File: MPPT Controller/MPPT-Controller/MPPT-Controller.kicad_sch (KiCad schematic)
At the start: 48 parts, among them J1 Conn_01x02_Pin, J2 Conn_01x02_Pin, J3 Conn_01x02_Pin, J4 USB_C_Receptacle_PowerOnly_6P, K1 JQC-3FF-005-1Z, Q1 BC817, U1 ADS1115IDGS, U2 ESP32-WROOM-32D

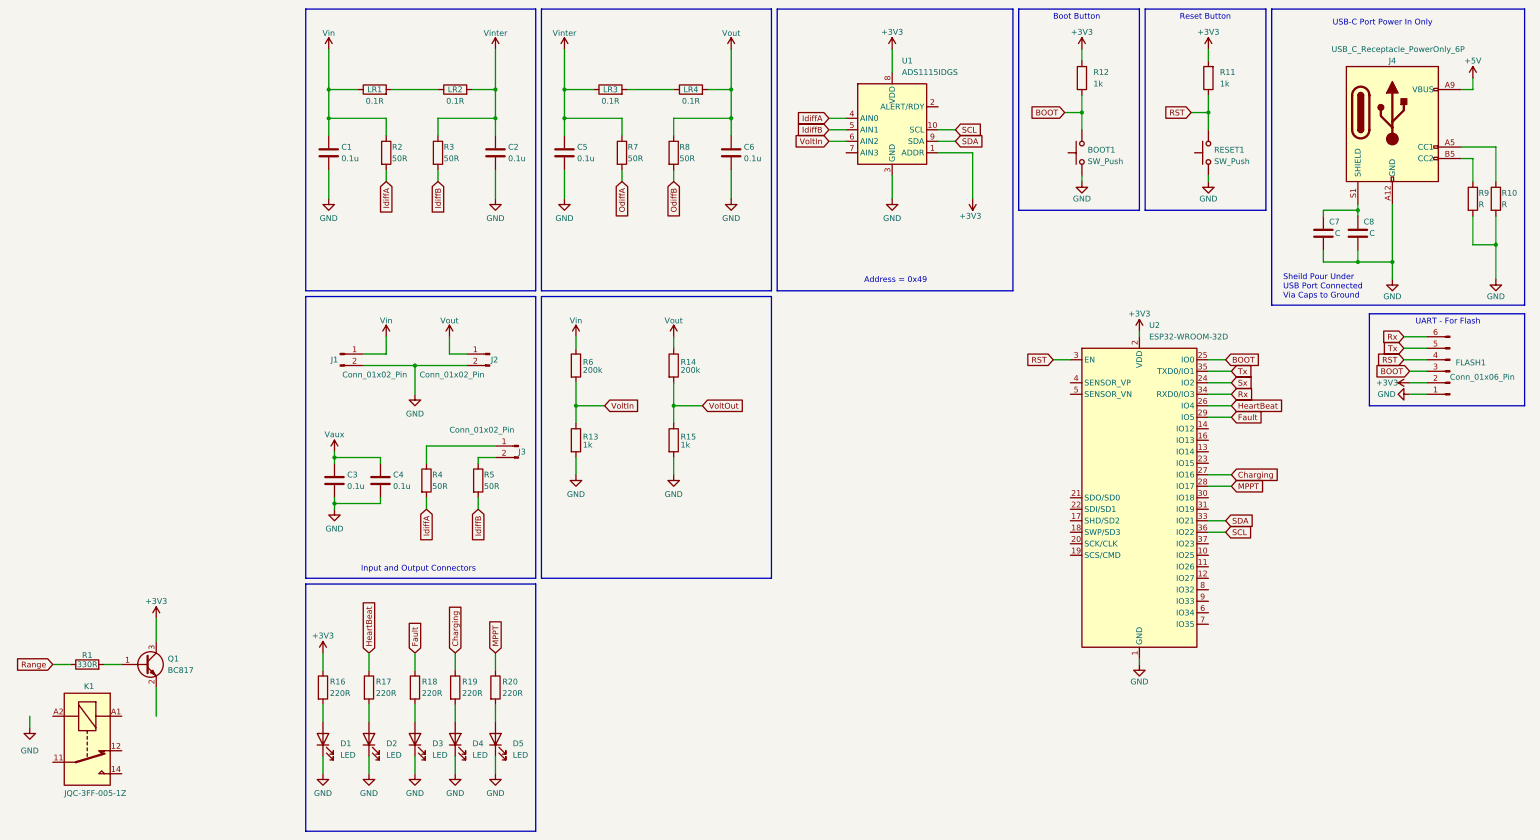
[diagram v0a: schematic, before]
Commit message: add
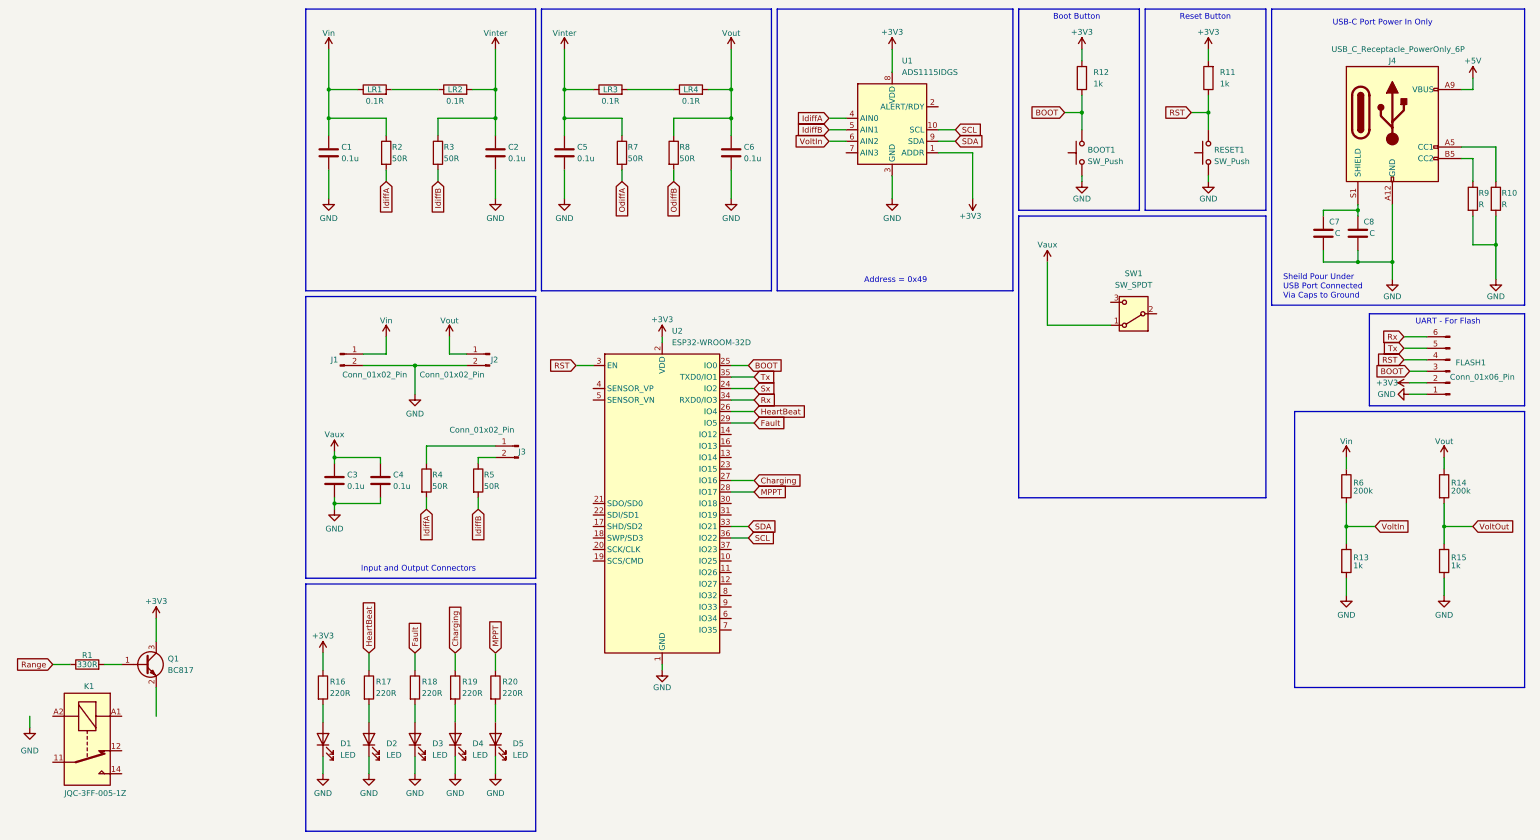
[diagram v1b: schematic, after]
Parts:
- added SW1: SW_SPDT, symbol Switch:SW_SPDT
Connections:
- net Vaux: now also SW1.1 (A)
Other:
- moved on the sheet: R13, R14, R15, R6, U2
